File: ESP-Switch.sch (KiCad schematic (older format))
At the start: 46 parts, among them J1 AC/In, K1 Relay, K2 Relay, K3 Relay, K4 Relay, Q1 BC817, Q2 BC817, Q3 BC817, Q4 BC817, U1 AMS1117-3.3, U2 ESP-01v090

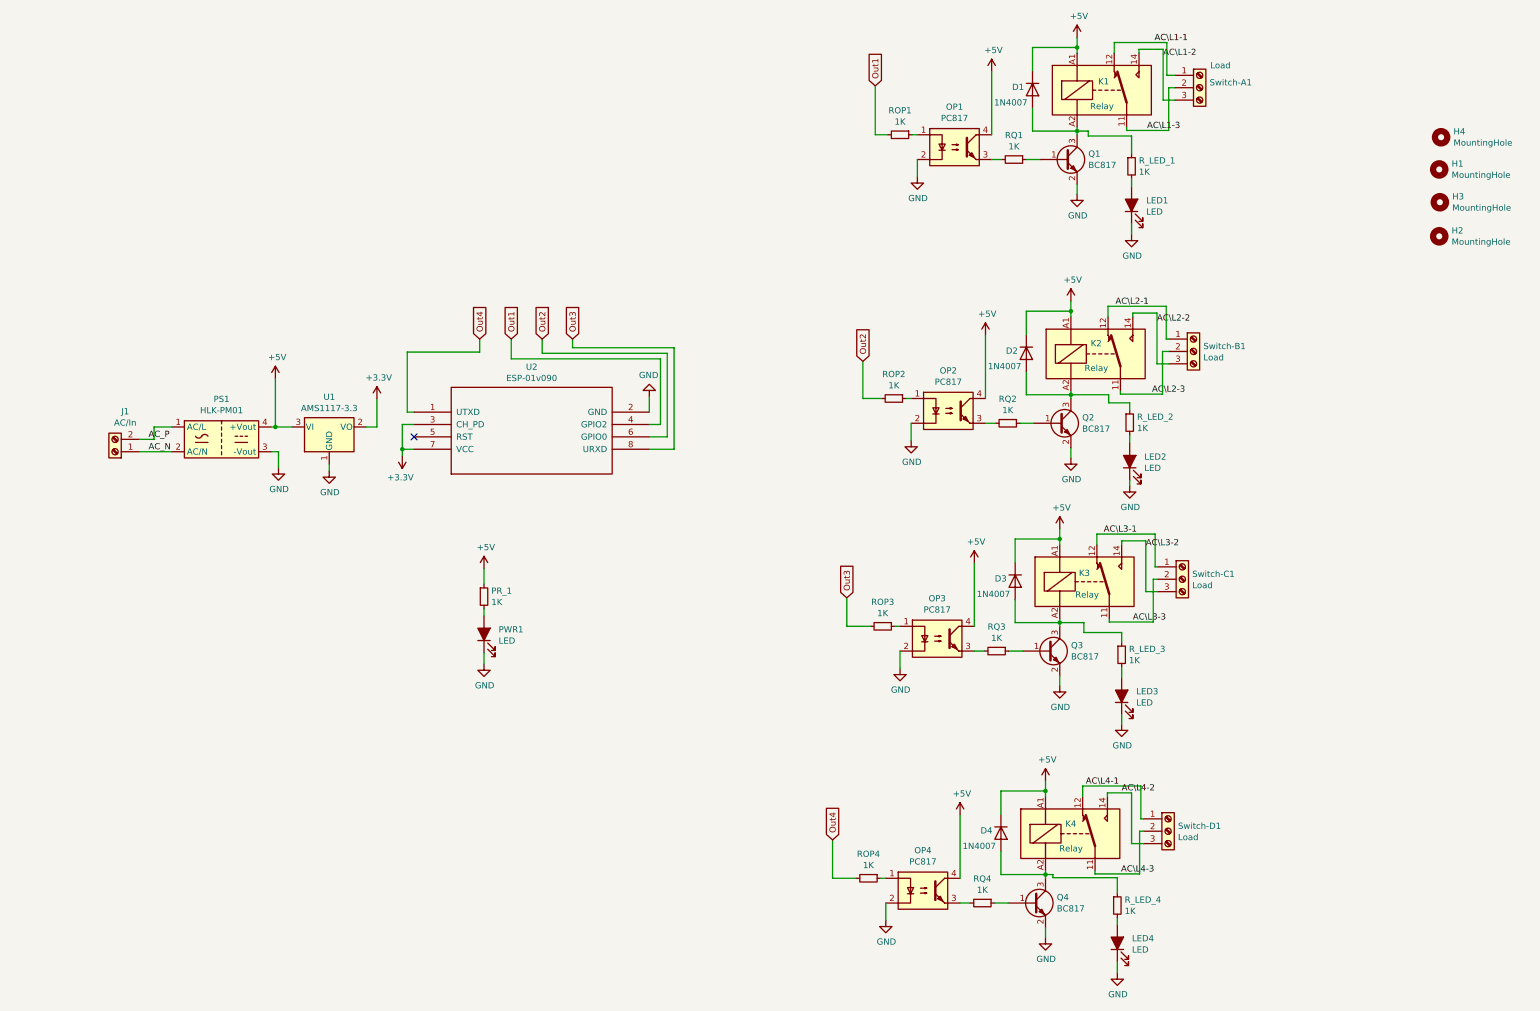
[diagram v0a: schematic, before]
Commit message: dimmer version
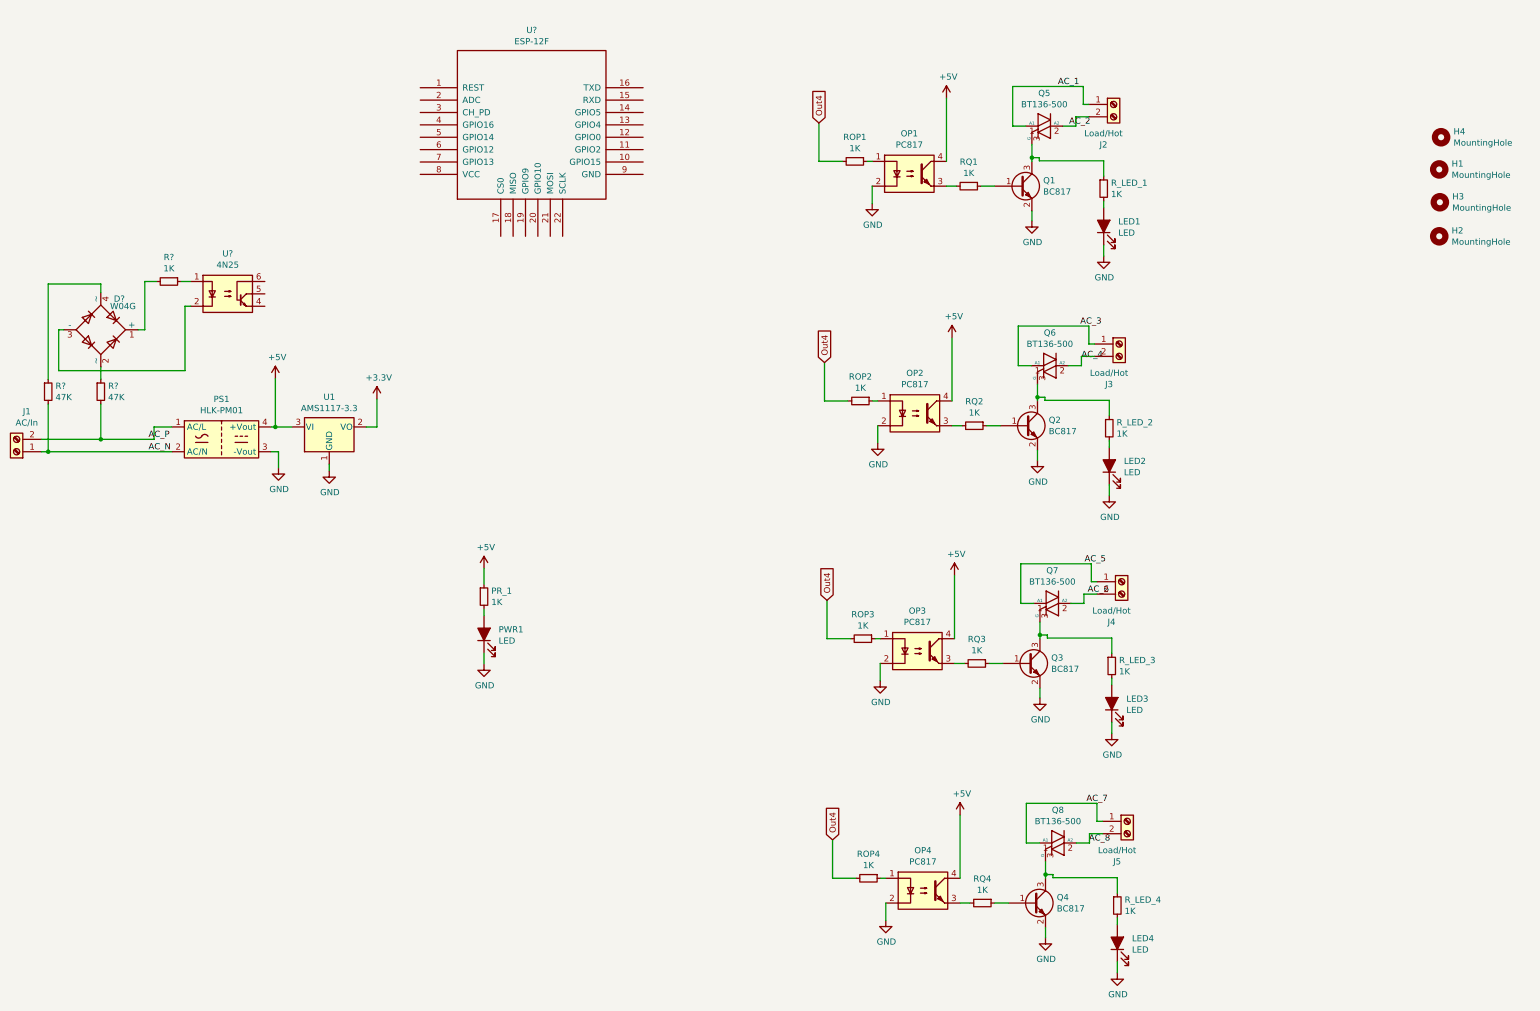
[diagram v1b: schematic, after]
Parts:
- removed D1, D2, D3, D4: 1N4007, Diode_SMD:D_SMA_Handsoldering, symbol Diode:1N4007
- removed K1, K2, K3, K4: Relay, Relay_THT:Relay_SPDT_Finder_36.11, symbol Relay:FINDER-36.11
- removed Switch-A1, Switch-B1, Switch-C1, Switch-D1: Load, TerminalBlock:TerminalBlock_Altech_AK300-3_P5.00mm, symbol Connector:Screw_Terminal_01x03
- removed U2: ESP-01v090, ESP:ESP-01, symbol ESP:ESP-01v090
- added D?: W04G, Diode_THT:Diode_Bridge_Round_D9.8mm, symbol Diode_Bridge:W04G
- added J2, J3, J4, J5: Load/Hot, TerminalBlock:TerminalBlock_Altech_AK300-2_P5.00mm, symbol Connector:Screw_Terminal_01x02
- added Q5, Q6, Q7, Q8: BT136-500, Package_TO_SOT_THT:TO-220-3_Vertical, symbol Triac_Thyristor:BT136-500
- added R? (x2): 47K, symbol Device:R_Small
- added R?: 1K, symbol Device:R_Small
- added U?: 4N25, Package_DIP:DIP-6_W7.62mm, symbol Isolator:4N25
- added U?: ESP-12F, symbol ESP:ESP-12F
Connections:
- net Out1 is gone; now on net Out4: ROP1.2
- net Out2 is gone; now on net Out4: ROP2.2
- net Out3 is gone; now on net Out4: ROP3.2
- net AC_N: now also R?.2
- net AC_P: now also R?.2
- net at Q2.3 (C), R_LED_2.1: now also Q6.3 (G)
- net at Q4.3 (C), R_LED_4.1: now also Q8.3 (G)
- net at Q3.3 (C), R_LED_3.1: now also Q7.3 (G)
- net at Q1.3 (C), R_LED_1.1: now also Q5.3 (G)
- new net: D?.1 (+), R?.2
- new net: D?.2 (~~), R?.1
- new net: D?.3 (-), U?.2
- new net: D?.4 (~~), R?.1
- new net: R?.1, U?.1
- new net AC_1: J2.1 (Pin_1), Q5.1 (A1)
- new net AC_2: J2.2 (Pin_2), Q5.2 (A2)
- new net AC_3: J3.1 (Pin_1), Q6.1 (A1)
- new net AC_4: J3.2 (Pin_2), Q6.2 (A2)
- new net AC_5: J4.1 (Pin_1), Q7.1 (A1)
- new net AC_6: J4.2 (Pin_2), Q7.2 (A2)
- new net AC_7: J5.1 (Pin_1), Q8.1 (A1)
- new net AC_8: J5.2 (Pin_2), Q8.2 (A2)
- no-connect marks 1 -> 0
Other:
- moved on the sheet: J1

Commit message: fixing the problems
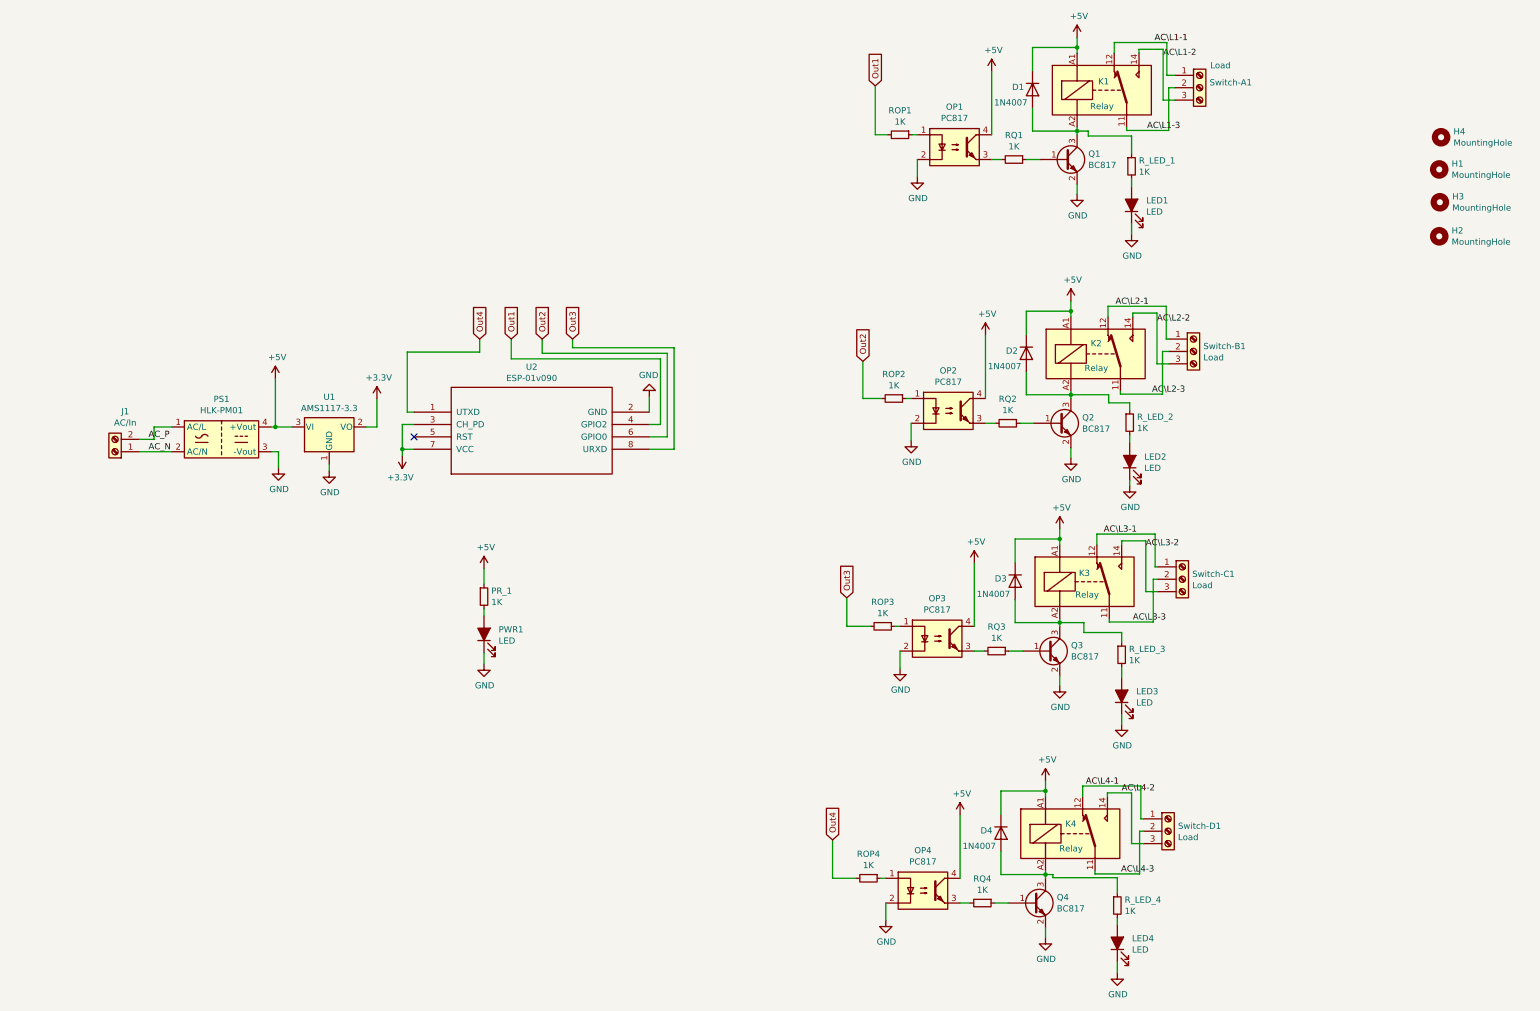
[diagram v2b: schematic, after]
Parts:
- removed D?: W04G, Diode_THT:Diode_Bridge_Round_D9.8mm, symbol Diode_Bridge:W04G
- removed J2, J3, J4, J5: Load/Hot, TerminalBlock:TerminalBlock_Altech_AK300-2_P5.00mm, symbol Connector:Screw_Terminal_01x02
- removed Q5, Q6, Q7, Q8: BT136-500, Package_TO_SOT_THT:TO-220-3_Vertical, symbol Triac_Thyristor:BT136-500
- removed R? (x2): 47K, symbol Device:R_Small
- removed R?: 1K, symbol Device:R_Small
- removed U?: 4N25, Package_DIP:DIP-6_W7.62mm, symbol Isolator:4N25
- removed U?: ESP-12F, symbol ESP:ESP-12F
- added D1, D2, D3, D4: 1N4007, Diode_SMD:D_SMA_Handsoldering, symbol Diode:1N4007
- added K1, K2, K3, K4: Relay, Relay_THT:Relay_SPDT_Finder_36.11, symbol Relay:FINDER-36.11
- added Switch-A1, Switch-B1, Switch-C1, Switch-D1: Load, TerminalBlock:TerminalBlock_Altech_AK300-3_P5.00mm, symbol Connector:Screw_Terminal_01x03
- added U2: ESP-01v090, ESP:ESP-01, symbol ESP:ESP-01v090
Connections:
- net +3V3: now also U2.3 (CH_PD), U2.7 (VCC)
- net +5V: now also D1.1 (K), D2.1 (K), D3.1 (K), D4.1 (K), K1.A1, K2.A1, K3.A1, K4.A1
- net GND: now also U2.2 (GND)
- net Out4: now also U2.1 (UTXD); no longer ROP1.2, ROP2.2, ROP3.2
- net at Q4.3 (C), R_LED_4.1: now also D4.2 (A), K4.A2
- net at Q3.3 (C), R_LED_3.1: now also D3.2 (A), K3.A2
- net at Q2.3 (C), R_LED_2.1: now also D2.2 (A), K2.A2
- net at Q1.3 (C), R_LED_1.1: now also D1.2 (A), K1.A2
- new net AC\L1-1: K1.12, Switch-A1.1 (Pin_1)
- new net AC\L1-2: K1.14, Switch-A1.3 (Pin_3)
- new net AC\L1-3: K1.11, Switch-A1.2 (Pin_2)
- new net AC\L2-1: K2.12, Switch-B1.1 (Pin_1)
- new net AC\L2-2: K2.14, Switch-B1.3 (Pin_3)
- new net AC\L2-3: K2.11, Switch-B1.2 (Pin_2)
- new net AC\L3-1: K3.12, Switch-C1.1 (Pin_1)
- new net AC\L3-2: K3.14, Switch-C1.3 (Pin_3)
- new net AC\L3-3: K3.11, Switch-C1.2 (Pin_2)
- new net AC\L4-1: K4.12, Switch-D1.1 (Pin_1)
- new net AC\L4-2: K4.14, Switch-D1.3 (Pin_3)
- new net AC\L4-3: K4.11, Switch-D1.2 (Pin_2)
- new net Out1: ROP1.2, U2.4 (GPIO2)
- new net Out2: ROP2.2, U2.6 (GPIO0)
- new net Out3: ROP3.2, U2.8 (URXD)
- no-connect marks 0 -> 1
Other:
- moved on the sheet: J1
